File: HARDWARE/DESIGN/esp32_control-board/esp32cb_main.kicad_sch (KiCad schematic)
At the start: 25 parts, among them J204 USB-prog, SW201 Boot, SW202 Reset, U203 ESP32-S3-WROOM-1U, U204 USBLC6-2SC6

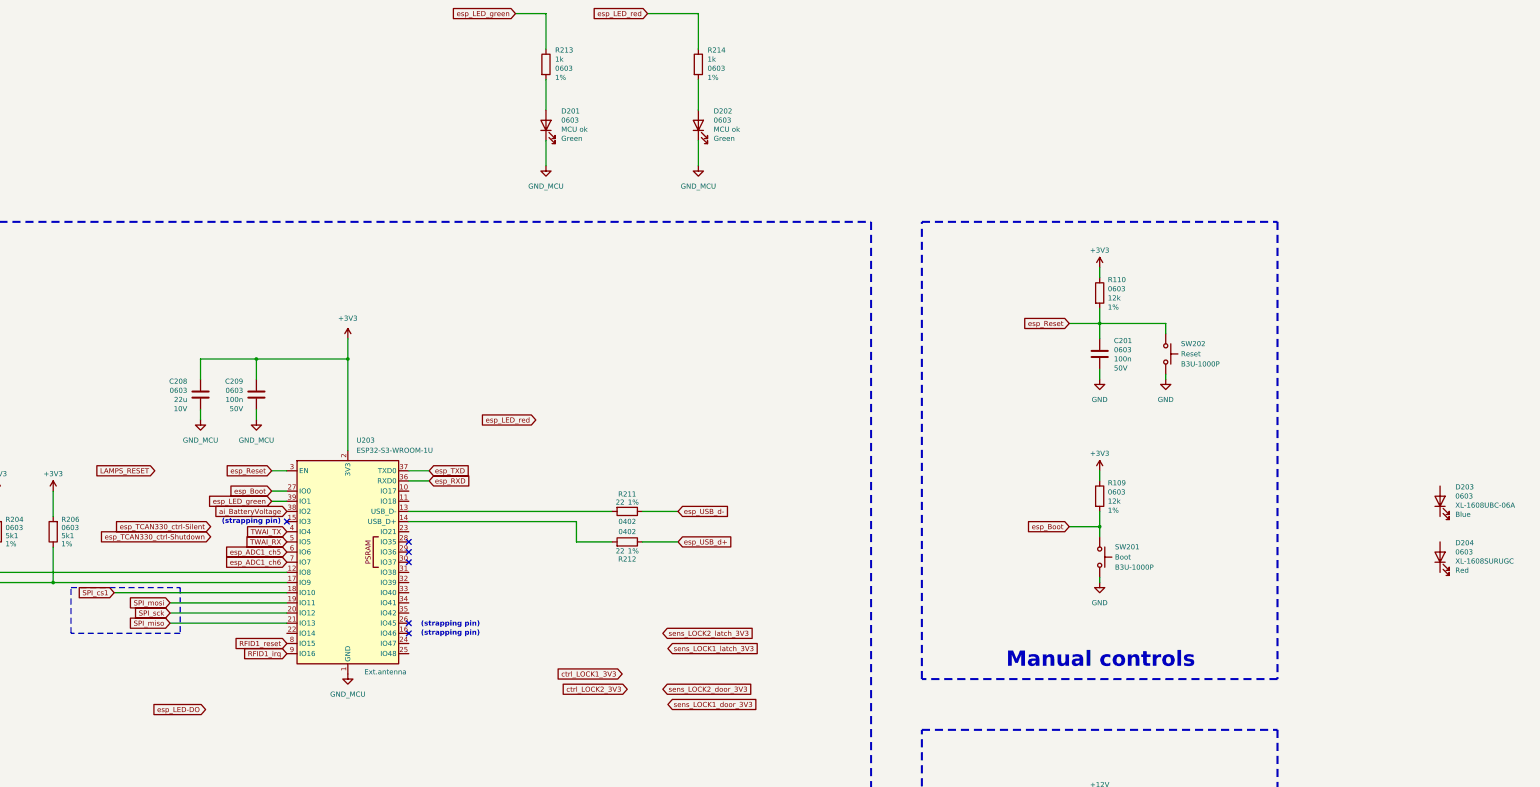
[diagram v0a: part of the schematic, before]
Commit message: 60911 - PCB-layout updated
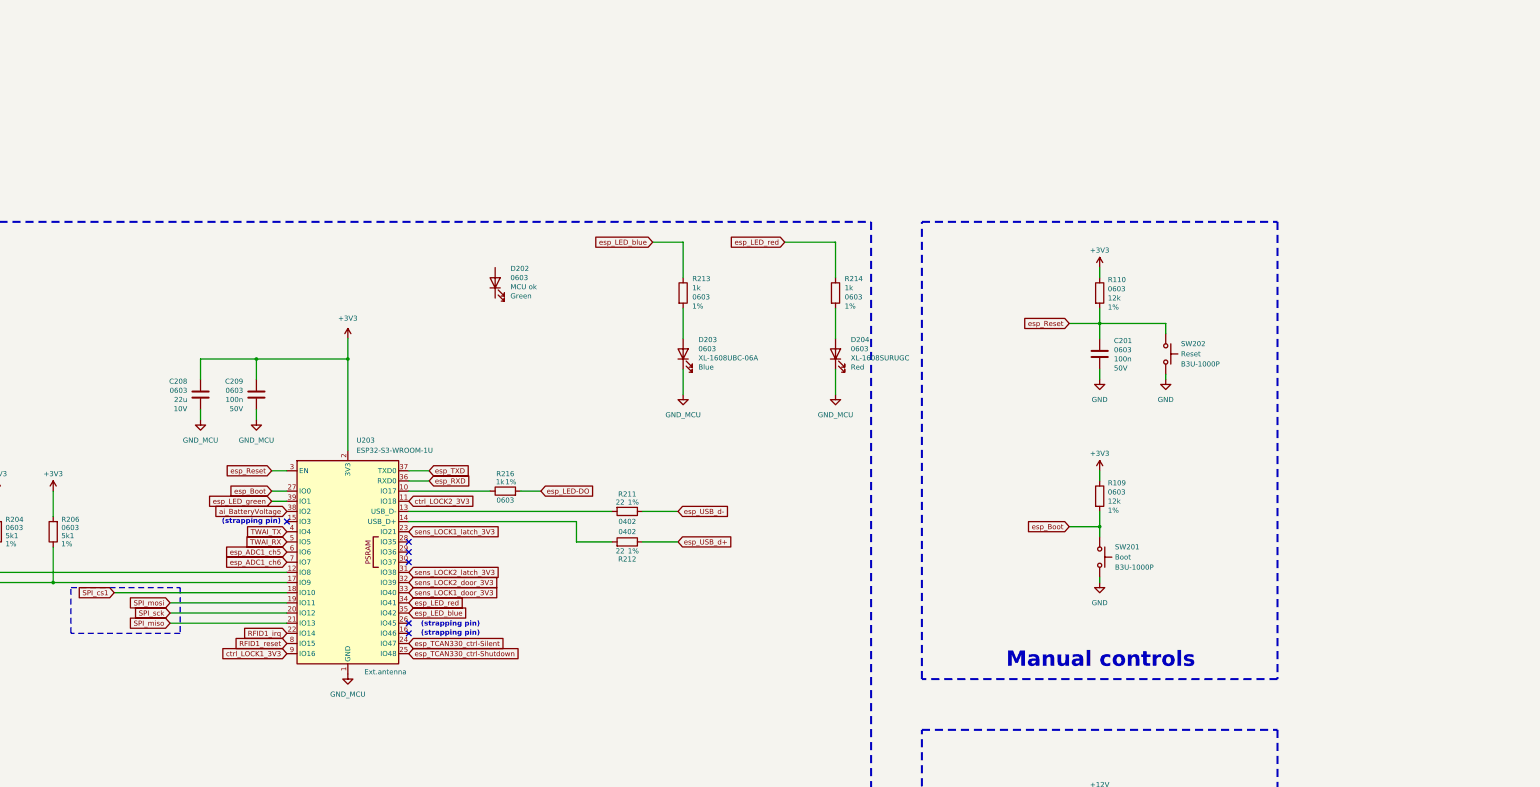
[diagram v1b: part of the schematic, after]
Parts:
- removed D201: MCU ok, LED_SMD:LED_0603_1608Metric, symbol Device:LED
- added R216: 1k, Resistor_SMD:R_0603_1608Metric, symbol Device:R
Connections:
- net GND_MCU: now also D203.1 (K), D204.1 (K); no longer D202.1 (K)
- net RFID1_irq: now also U203.22 (IO14); no longer U203.9 (IO16)
- net ctrl_LOCK1_3V3: now also U203.9 (IO16)
- net ctrl_LOCK2_3V3: now also U203.11 (IO18)
- net esp_LED-DO: now also R216.2
- net esp_LED_green: no longer R213.1
- net esp_LED_red: now also U203.34 (IO41)
- net esp_TCAN330_ctrl-Shutdown: now also U203.25 (IO48)
- net esp_TCAN330_ctrl-Silent: now also U203.24 (IO47)
- net sens_LOCK1_door_3V3: now also U203.33 (IO40)
- net sens_LOCK1_latch_3V3: now also U203.23 (IO21)
- net sens_LOCK2_door_3V3: now also U203.32 (IO39)
- net sens_LOCK2_latch_3V3: now also U203.31 (IO38)
- net at R214.2: now also D204.2 (A); no longer D202.2 (A)
- net at R213.2: now also D203.2 (A)
- net at U203.10 (IO17): now also R216.1
- net esp_LED_blue: now reaches U203.35 (IO42)
- net esp_LED_blue: now also R213.1
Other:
- moved on the sheet: D203, D204, R213, R214

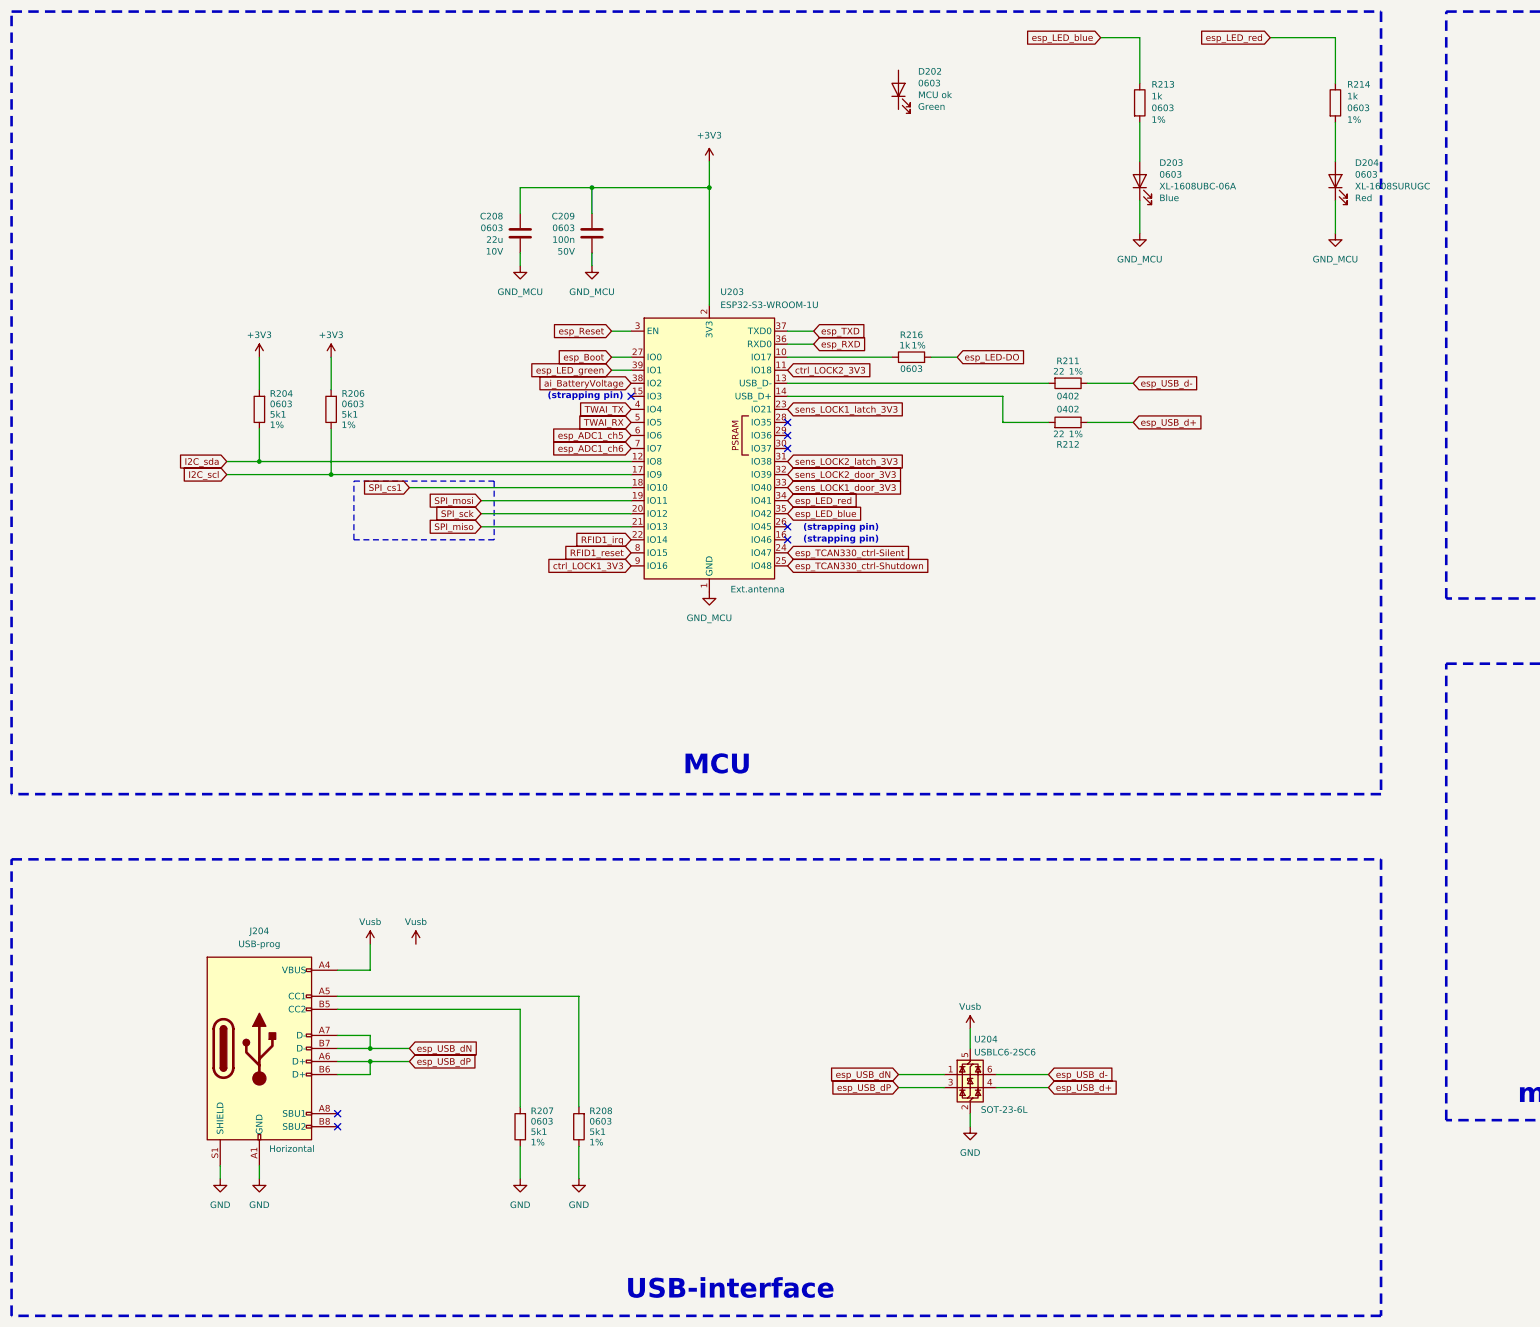
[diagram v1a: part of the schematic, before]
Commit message: 60911 - Schematic minor update
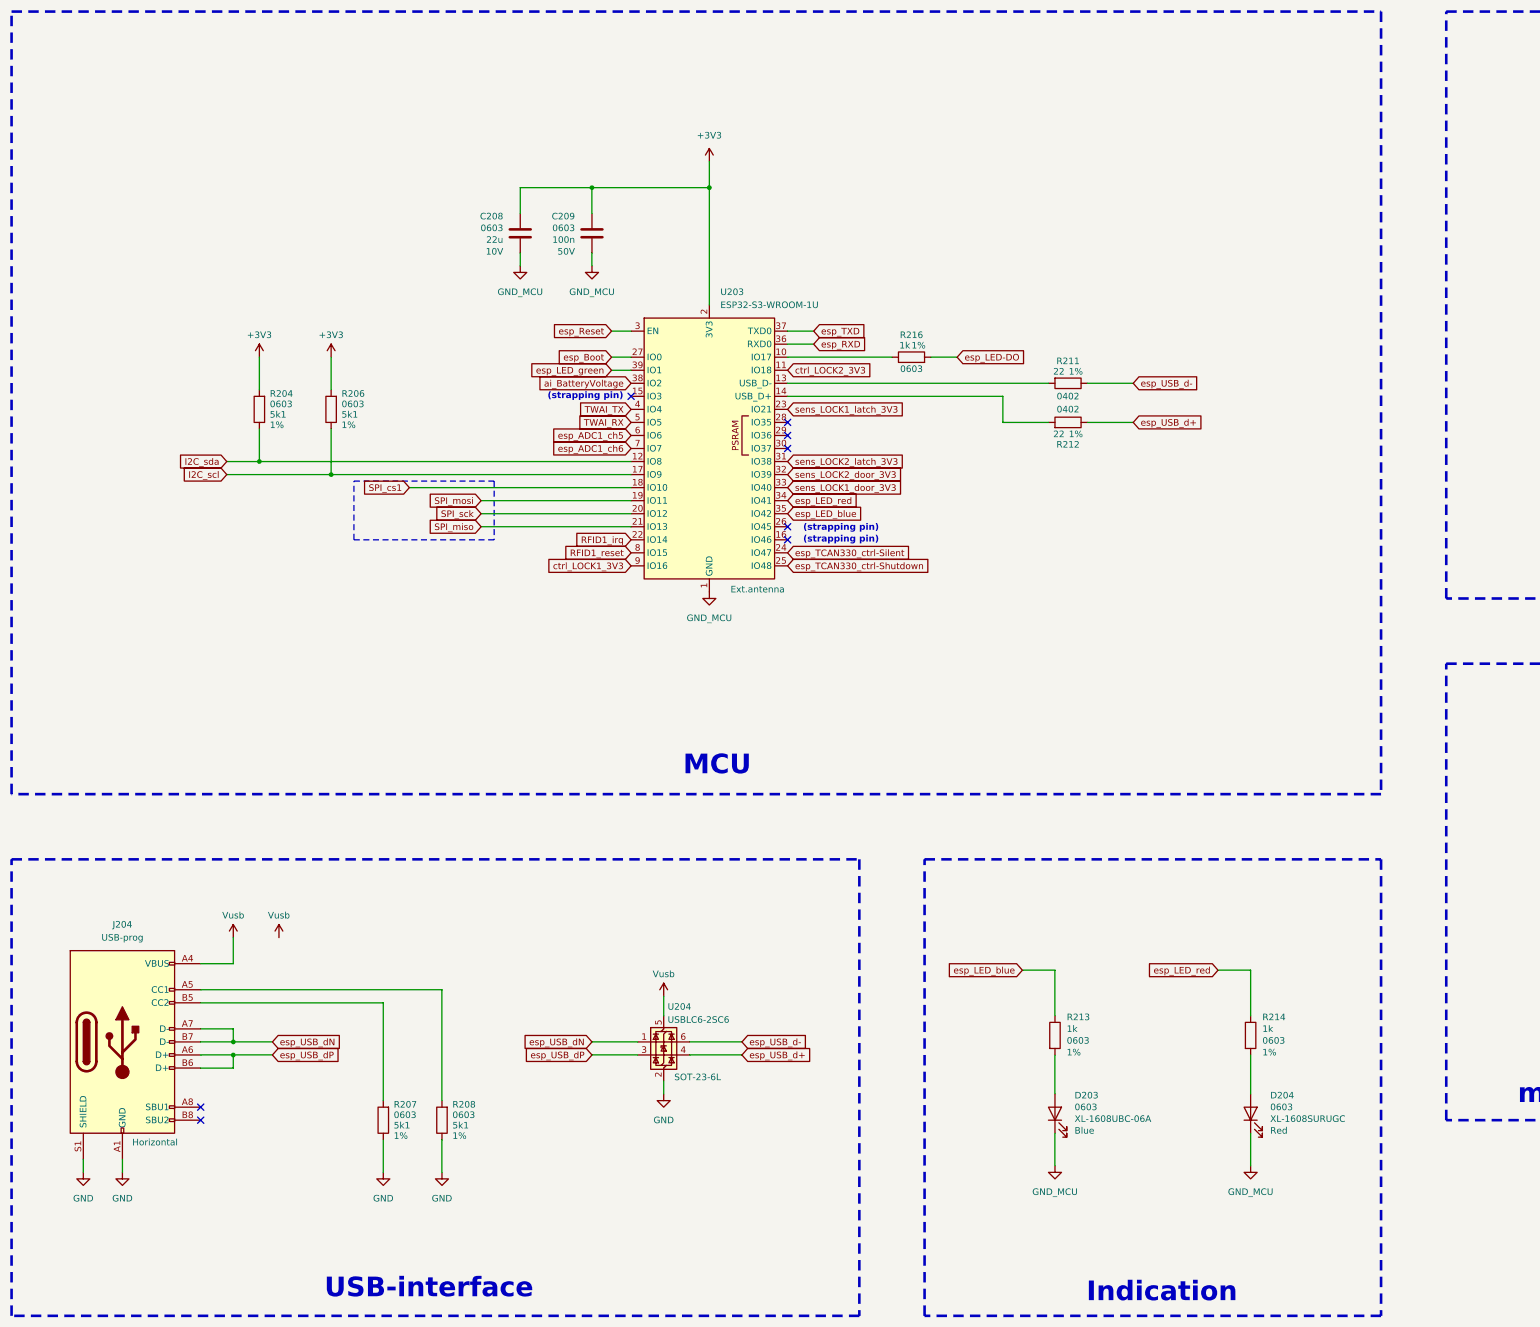
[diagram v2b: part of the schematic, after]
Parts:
- removed D202: MCU ok, LED_SMD:LED_0603_1608Metric, symbol Device:LED
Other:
- note added: "Indication"
- moved on the sheet: D203, D204, J204, R207, R208, R213, R214, U204
